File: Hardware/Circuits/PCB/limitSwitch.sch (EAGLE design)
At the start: 25 parts

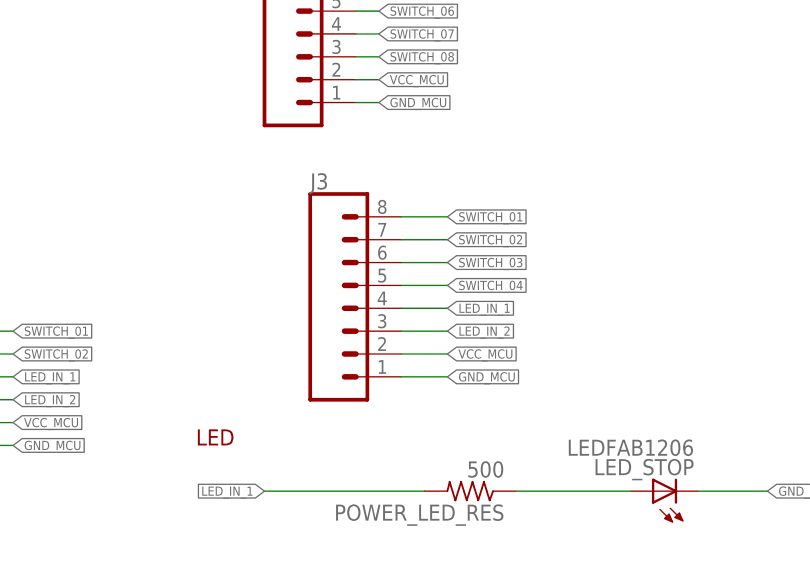
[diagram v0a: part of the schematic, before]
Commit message: update circuits
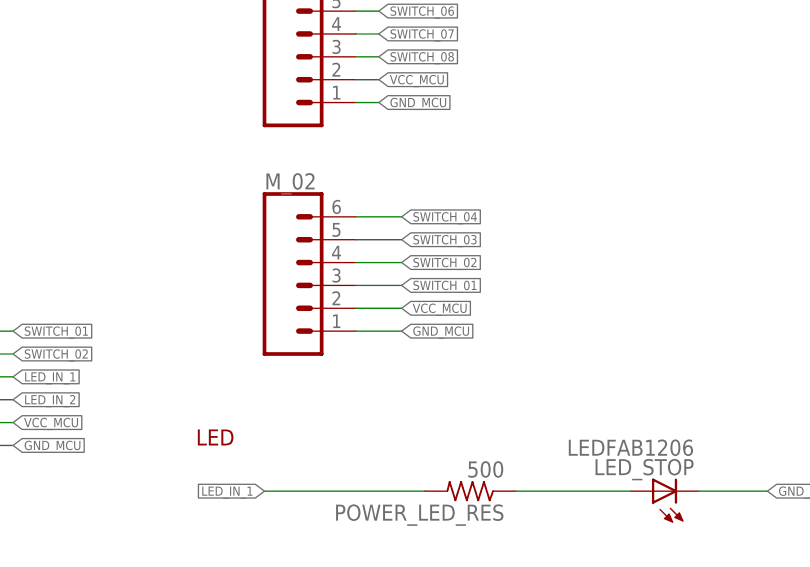
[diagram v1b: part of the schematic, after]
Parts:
- removed J3: (no value), SparkFun-Connectors:CONN_08BM08B-SRSS-TB
- added M_02: (no value), SparkFun-Connectors:CONN_06SMD-1MM
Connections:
- net GND_MCU: now also M_02.1; no longer J3.1
- net LED_IN_1: no longer J3.4
- net LED_IN_2: no longer J3.3
- net SWITCH_01: now also M_02.3; no longer J3.8
- net SWITCH_02: now also M_02.4; no longer J3.7
- net SWITCH_03: now also M_02.5; no longer J3.6
- net SWITCH_04: now also M_02.6; no longer J3.5
- net VCC_MCU: now also M_02.2; no longer J3.2
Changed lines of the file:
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@@
 <clearance class="0" value="0.2"/>
 </class>
-<class number="1" name="New Class" width="0.2" drill="0">
-<clearance class="1" value="0.00508125"/>
+<class number="1" name="New Class" width="0.4" drill="0">
+<clearance class="1" value="0.2"/>
 </class>
 </classes>
@@
 <part name="R8" library="resistor" library_urn="urn:adsk.eagle:library:348" deviceset="R-US_" device="M0805" package3d_urn="urn:adsk.eagle:package:26079/1" value="10k"/>
 <part name="SWITCH_M8" library="switch-tact" deviceset="DTSM-3" device=""/>
-<part name="J3" library="SparkFun-Connectors" library_urn="urn:adsk.eagle:library:513" deviceset="CONN_08" device="BM08B-SRSS-TB" package3d_urn="urn:adsk.eagle:package:38145/1"/>
+<part name="M_02" library="SparkFun-Connectors" library_urn="urn:adsk.eagle:library:513" deviceset="CONN_06" device="SMD-1MM" package3d_urn="urn:adsk.eagle:package:38023/1"/>
 </parts>
 <sheets>
@@
 <attribute name="VALUE" x="330.835" y="52.07" size="1.778" layer="96"/>
 </instance>
-<instance part="J3" gate="G$1" x="73.66" y="63.5" smashed="yes">
-<attribute name="VALUE" x="68.58" y="51.054" size="1.778" layer="96" font="vector"/>
-<attribute name="NAME" x="68.58" y="76.708" size="1.778" layer="95" font="vector"/>
+<instance part="M_02" gate="G$1" x="68.58" y="66.04" smashed="yes">
+<attribute name="VALUE" x="63.5" y="56.134" size="1.778" layer="96" font="vector"/>
+<attribute name="NAME" x="63.5" y="76.708" size="1.778" layer="95" font="vector"/>
 </instance>
 </instances>
@@
 </segment>
 <segment>
-<pinref part="J3" gate="G$1" pin="7"/>
-<wire x1="78.74" y1="71.12" x2="83.82" y2="71.12" width="0.1524" layer="91"/>
-<label x="83.82" y="71.12" size="1.016" layer="95" xref="yes"/>
+<pinref part="M_02" gate="G$1" pin="4"/>
+<wire x1="73.66" y1="68.58" x2="78.74" y2="68.58" width="0.1524" layer="91"/>
+<label x="78.74" y="68.58" size="1.016" layer="95" xref="yes"/>
 </segment>
 </net>
@@
 </segment>
 <segment>
-<pinref part="J3" gate="G$1" pin="1"/>
-<wire x1="78.74" y1="55.88" x2="83.82" y2="55.88" width="0.1524" layer="91"/>
-<label x="83.82" y="55.88" size="1.016" layer="95" xref="yes"/>
+<pinref part="M_02" gate="G$1" pin="1"/>
+<wire x1="73.66" y1="60.96" x2="78.74" y2="60.96" width="0.1524" layer="91"/>
+<label x="78.74" y="60.96" size="1.016" layer="95" xref="yes"/>
 </segment>
 </net>
@@
 </segment>
 <segment>
-<pinref part="J3" gate="G$1" pin="2"/>
-<wire x1="78.74" y1="58.42" x2="83.82" y2="58.42" width="0.1524" layer="91"/>
-<label x="83.82" y="58.42" size="1.016" layer="95" xref="yes"/>
+<pinref part="M_02" gate="G$1" pin="2"/>
+<wire x1="73.66" y1="63.5" x2="78.74" y2="63.5" width="0.1524" layer="91"/>
+<label x="78.74" y="63.5" size="1.016" layer="95" xref="yes"/>
 </segment>
 </net>
@@
 <wire x1="149.86" y1="22.86" x2="142.24" y2="22.86" width="0.1524" layer="91"/>
 <label x="142.24" y="22.86" size="1.016" layer="95" rot="R180" xref="yes"/>
-</segment>
-<segment>
-<pinref part="J3" gate="G$1" pin="3"/>
-<wire x1="78.74" y1="60.96" x2="83.82" y2="60.96" width="0.1524" layer="91"/>
-<label x="83.82" y="60.96" size="1.016" layer="95" xref="yes"/>
 </segment>
 </net>
@@
 </segment>
 <segment>
-<pinref part="J3" gate="G$1" pin="8"/>
-<wire x1="78.74" y1="73.66" x2="83.82" y2="73.66" width="0.1524" layer="91"/>
-<label x="83.82" y="73.66" size="1.016" layer="95" xref="yes"/>
+<pinref part="M_02" gate="G$1" pin="3"/>
+<wire x1="73.66" y1="66.04" x2="78.74" y2="66.04" width="0.1524" layer="91"/>
+<label x="78.74" y="66.04" size="1.016" layer="95" xref="yes"/>
 </segment>
 </net>
@@
 </segment>
 <segment>
-<pinref part="J3" gate="G$1" pin="5"/>
-<wire x1="78.74" y1="66.04" x2="83.82" y2="66.04" width="0.1524" layer="91"/>
-<label x="83.82" y="66.04" size="1.016" layer="95" xref="yes"/>
+<pinref part="M_02" gate="G$1" pin="6"/>
+<wire x1="73.66" y1="73.66" x2="78.74" y2="73.66" width="0.1524" layer="91"/>
+<label x="78.74" y="73.66" size="1.016" layer="95" xref="yes"/>
 </segment>
 </net>
@@
 </segment>
 <segment>
-<pinref part="J3" gate="G$1" pin="6"/>
-<wire x1="78.74" y1="68.58" x2="83.82" y2="68.58" width="0.1524" layer="91"/>
-<label x="83.82" y="68.58" size="1.016" layer="95" xref="yes"/>
+<pinref part="M_02" gate="G$1" pin="5"/>
+<wire x1="73.66" y1="71.12" x2="78.74" y2="71.12" width="0.1524" layer="91"/>
+<label x="78.74" y="71.12" size="1.016" layer="95" xref="yes"/>
 </segment>
 </net>
@@
 <wire x1="149.86" y1="43.18" x2="142.24" y2="43.18" width="0.1524" layer="91"/>
 <label x="142.24" y="43.18" size="1.016" layer="95" rot="R180" xref="yes"/>
-</segment>
-<segment>
-<pinref part="J3" gate="G$1" pin="4"/>
-<wire x1="78.74" y1="63.5" x2="83.82" y2="63.5" width="0.1524" layer="91"/>
-<label x="83.82" y="63.5" size="1.016" layer="95" xref="yes"/>
 </segment>
 </net>
@@
 </sheet>
 </sheets>
+<errors>
+</errors>
 </schematic>
 </drawing>
